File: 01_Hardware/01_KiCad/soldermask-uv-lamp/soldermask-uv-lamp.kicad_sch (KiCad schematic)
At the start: 12 parts, among them J1 USB_C_Receptacle_USB2.0_16P, Q1 BC817

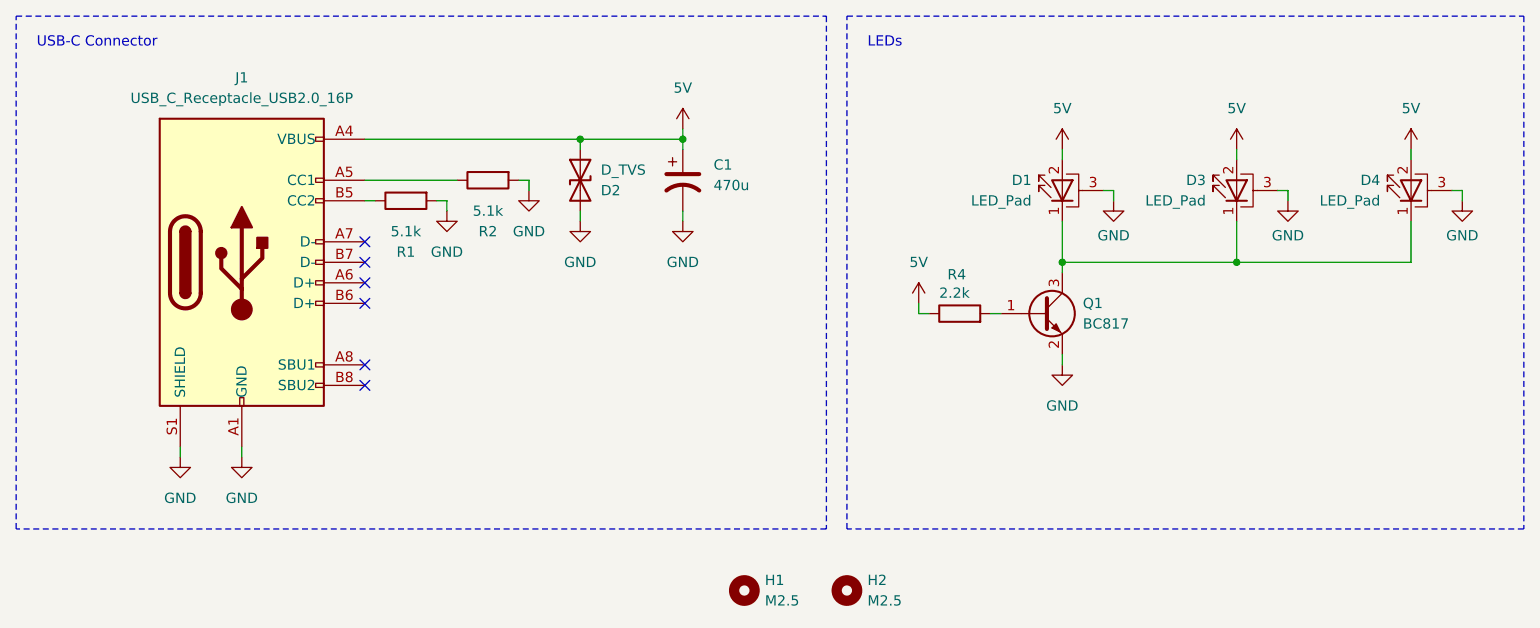
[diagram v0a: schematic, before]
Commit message: Repo cleanup: gitignore, README, license, optimized renders
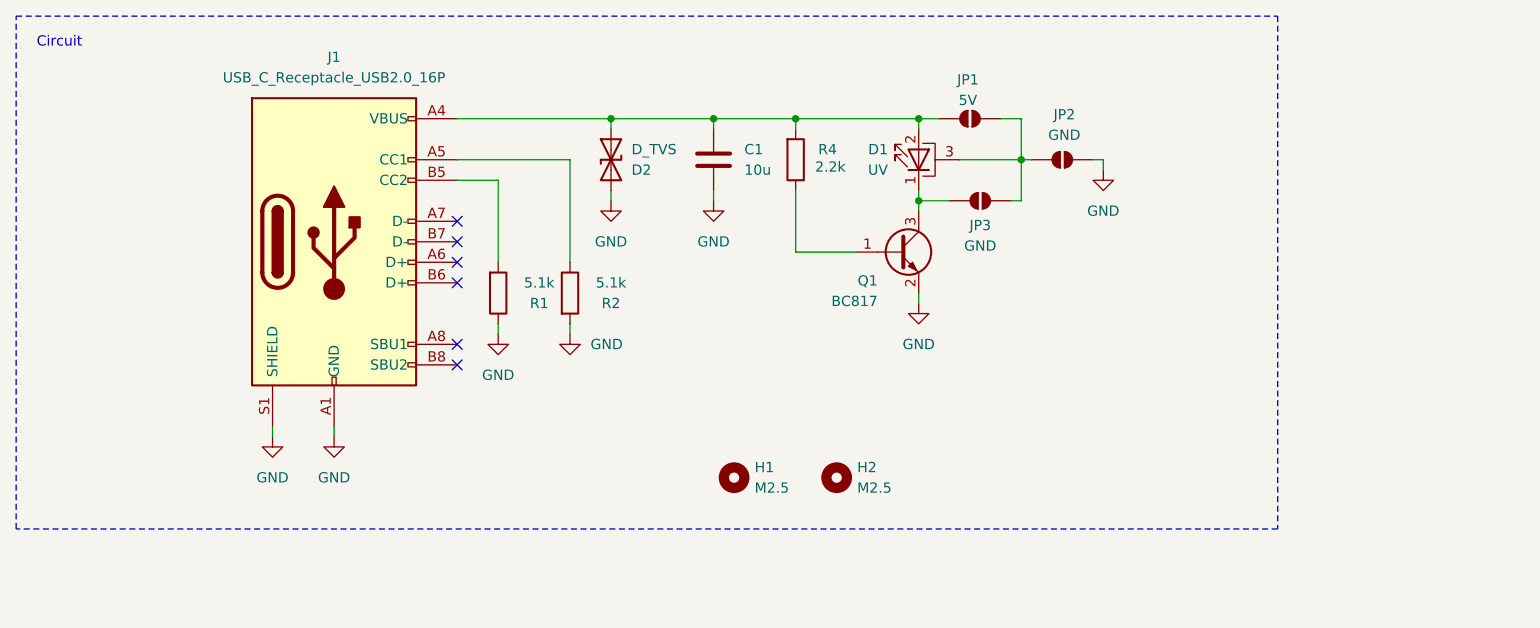
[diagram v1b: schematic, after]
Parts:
- removed C1: 470u, Capacitor_SMD:CP_Elec_8x10, symbol Device:C_Polarized_US
- removed D3, D4: LED_Pad, LED_SMD:LED_Cree-XHP35, symbol Device:LED_Pad
- added C1: 10u, Capacitor_SMD:C_1206_3216Metric, symbol Device:C
- added JP1: 5V, Jumper:SolderJumper-2_P1.3mm_Open_RoundedPad1.0x1.5mm, symbol Jumper:SolderJumper_2_Open
- added JP2, JP3: GND, Jumper:SolderJumper-2_P1.3mm_Open_RoundedPad1.0x1.5mm, symbol Jumper:SolderJumper_2_Open
- D1: value LED_Pad -> UV; footprint LED_SMD:LED_Cree-XHP35 -> LED_SMD:LED_1W_3W_R8; TME https://www.tme.eu/pl/details/pk2n-1kqe-sl/diody-led-uv/pro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 -> https://www.tme.eu/pl/details/osv3xme3e1e/diody-led-uv/opto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
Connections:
- net GND: now also R1.1, C1.2, JP2.1 (A); no longer D1.3 (PAD), R1.2
- net at D1.1 (K), Q1.3 (C): now also JP3.1 (A)
- net at R4.2: now also D1.2 (A), D2.1 (A1), J1.A4 (VBUS), J1.A9 (VBUS), J1.B4 (VBUS), J1.B9 (VBUS), C1.1, JP1.1 (A); no longer Q1.1 (B)
- net at J1.B5 (CC2): now also R1.2; no longer R1.1
- removed net 5V: D1.2 (A), D2.1 (A1), J1.A4 (VBUS), J1.A9 (VBUS), J1.B4 (VBUS), J1.B9 (VBUS), R4.1
- new net: D1.3 (PAD), JP1.2 (B), JP2.2 (B), JP3.2 (B)
- new net: Q1.1 (B), R4.1
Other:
- note added: "Circuit"
- note removed: "LEDs"
- note removed: "USB-C Connector"
- moved on the sheet: D2, H1, H2, J1, Q1, R2, R4
